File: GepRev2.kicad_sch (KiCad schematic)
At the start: 194 parts

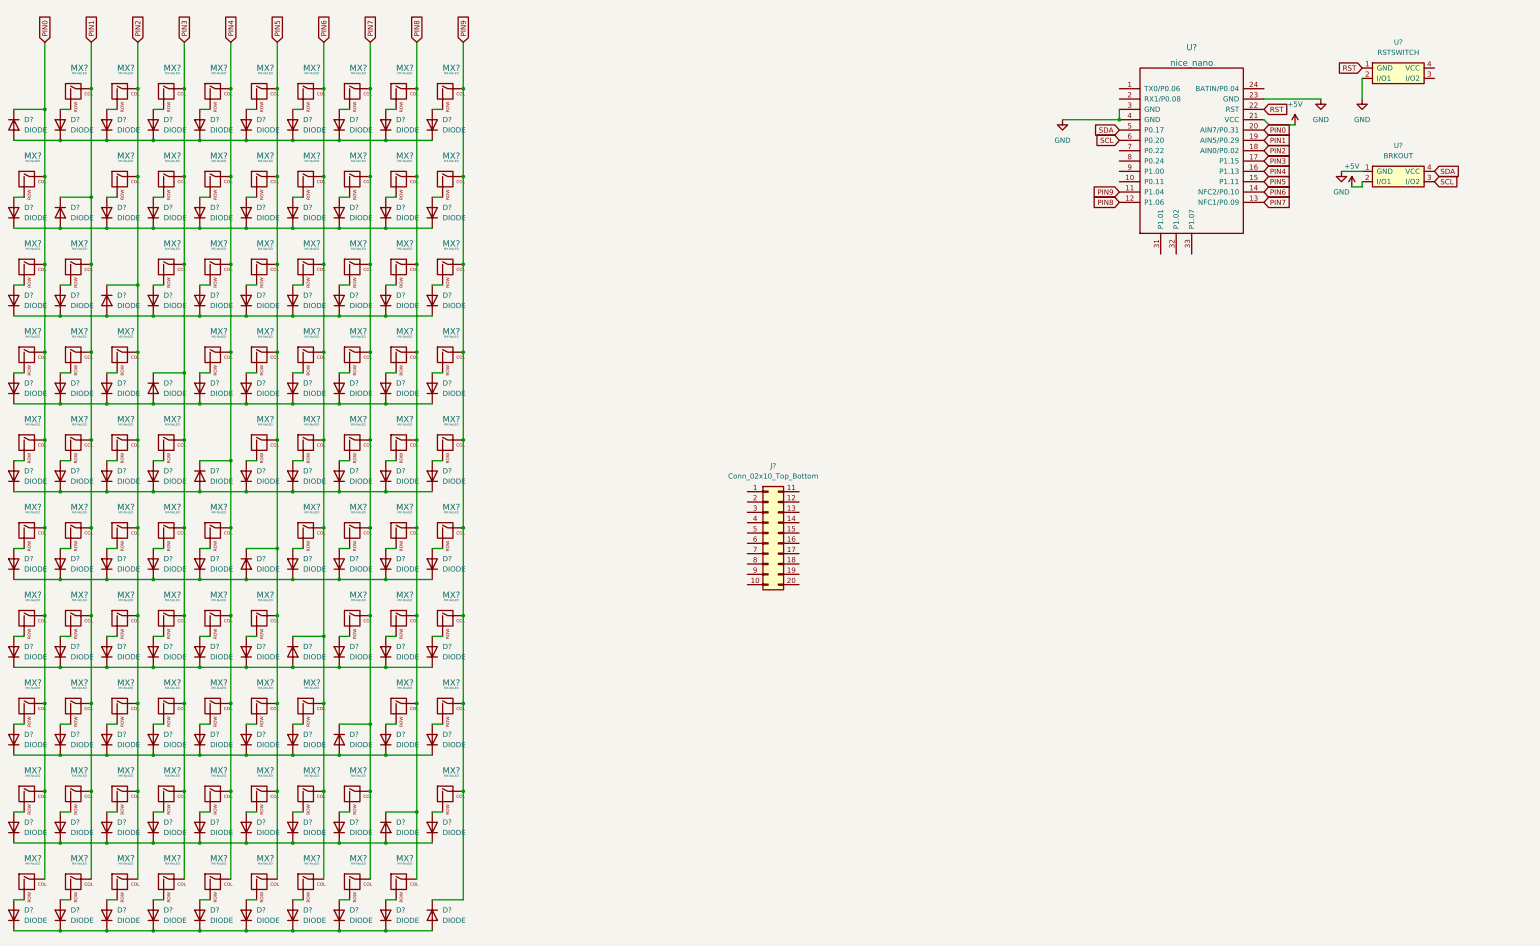
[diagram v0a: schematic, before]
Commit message: Updates to schematic
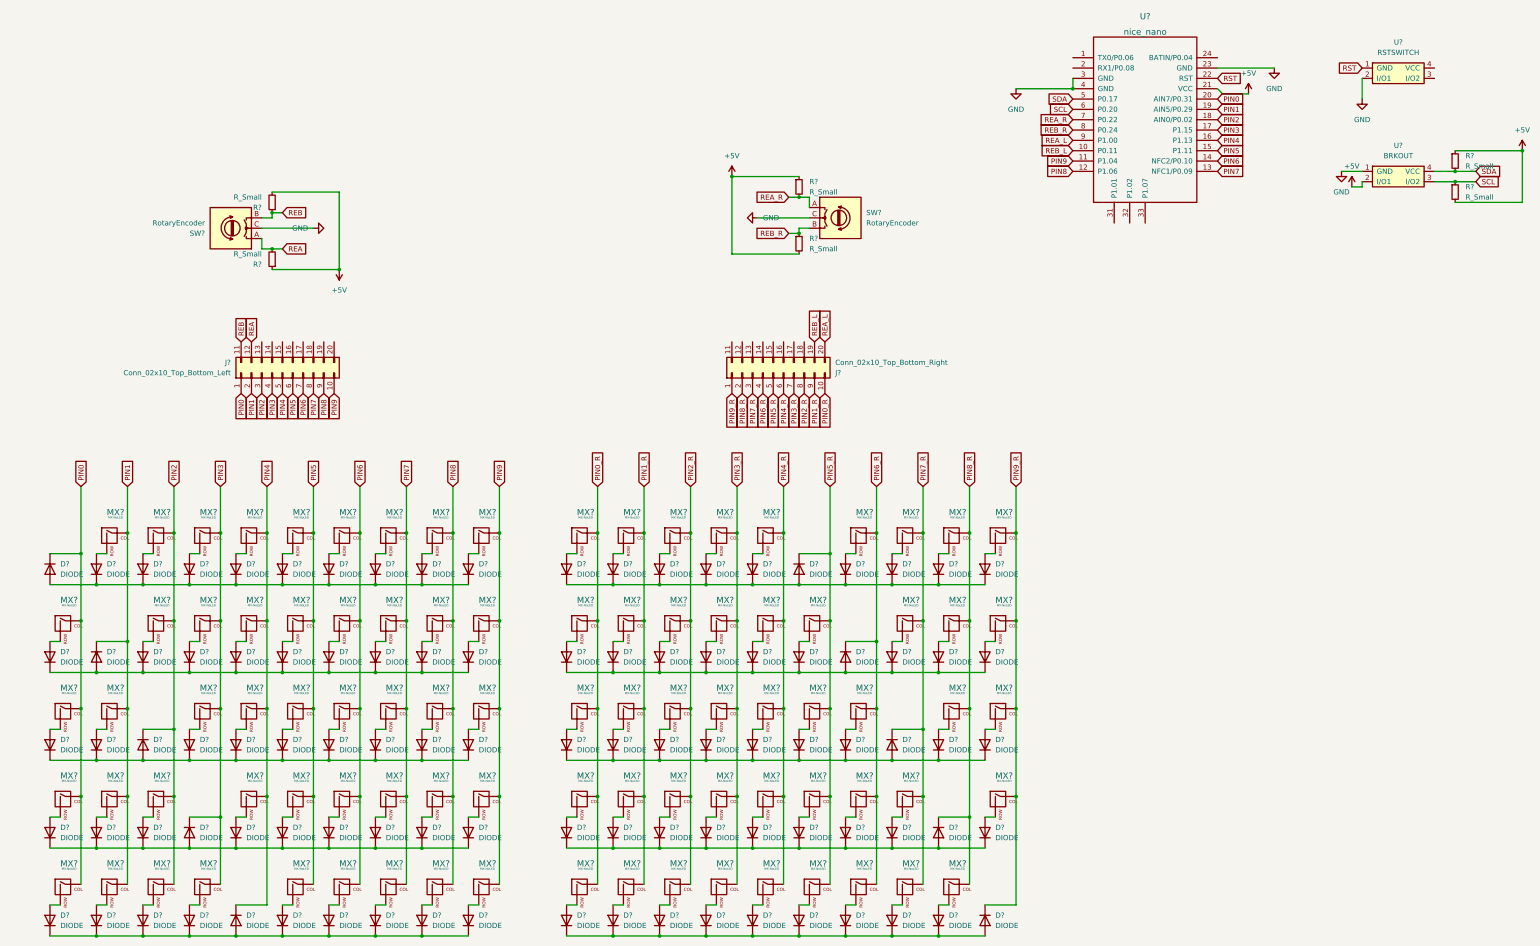
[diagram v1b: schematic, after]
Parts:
- added J?: Conn_02x10_Top_Bottom_Left, symbol Connector_Generic:Conn_02x10_Top_Bottom
- added R? (x6): R_Small, symbol Device:R_Small
- added SW? (x2): RotaryEncoder, symbol Device:RotaryEncoder
- J?: value Conn_02x10_Top_Bottom -> Conn_02x10_Top_Bottom_Right
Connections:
- net +5V: now also R?.1, R?.1, R?.1, R?.2, R?.2, R?.2
- net GND: now also SW?.C, SW?.C
- net PIN0: now also J?.1 (Pin_1); no longer MX?.1 (COL), MX?.1 (COL), MX?.1 (COL), MX?.1 (COL), MX?.1 (COL)
- net PIN1: now also J?.2 (Pin_2); no longer MX?.1 (COL), MX?.1 (COL), MX?.1 (COL), MX?.1 (COL), MX?.1 (COL)
- net PIN2: now also J?.3 (Pin_3); no longer MX?.1 (COL), MX?.1 (COL), MX?.1 (COL), MX?.1 (COL), MX?.1 (COL)
- net PIN3: now also J?.4 (Pin_4); no longer MX?.1 (COL), MX?.1 (COL), MX?.1 (COL), MX?.1 (COL), MX?.1 (COL)
- net PIN4: now also J?.5 (Pin_5); no longer MX?.1 (COL), MX?.1 (COL), MX?.1 (COL), MX?.1 (COL), MX?.1 (COL)
- net PIN5: now also J?.6 (Pin_6); no longer D?.2 (K), MX?.1 (COL), MX?.1 (COL), MX?.1 (COL), MX?.1 (COL)
- net PIN6: now also J?.7 (Pin_7); no longer D?.2 (K), MX?.1 (COL), MX?.1 (COL), MX?.1 (COL), MX?.1 (COL)
- net PIN7: now also J?.8 (Pin_8); no longer D?.2 (K), MX?.1 (COL), MX?.1 (COL), MX?.1 (COL), MX?.1 (COL)
- net PIN8: now also J?.9 (Pin_9); no longer D?.2 (K), MX?.1 (COL), MX?.1 (COL), MX?.1 (COL), MX?.1 (COL)
- net PIN9: now also J?.10 (Pin_10); no longer D?.2 (K), MX?.1 (COL), MX?.1 (COL), MX?.1 (COL), MX?.1 (COL)
- net SCL: now also R?.1
- net SDA: now also R?.2
- net REB_L: now reaches U?.10 (P0.11)
- net REB_L: now also J?.19 (Pin_19)
- net REA_R: now reaches U?.7 (P0.22)
- net REA_R: now also R?.2, SW?.A
- net REB_R: now reaches U?.8 (P0.24)
- net REB_R: now also R?.1, SW?.B
- net REA_L: now reaches U?.9 (P1.00)
- net REA_L: now also J?.20 (Pin_20)
- net PIN9_R: now reaches J?.1 (Pin_1)
- net PIN9_R: now also D?.2 (K), MX?.1 (COL), MX?.1 (COL), MX?.1 (COL), MX?.1 (COL)
- net PIN0_R: now reaches J?.10 (Pin_10)
- net PIN0_R: now also MX?.1 (COL), MX?.1 (COL), MX?.1 (COL), MX?.1 (COL), MX?.1 (COL)
- net PIN8_R: now reaches J?.2 (Pin_2)
- net PIN8_R: now also D?.2 (K), MX?.1 (COL), MX?.1 (COL), MX?.1 (COL), MX?.1 (COL)
- net PIN7_R: now reaches J?.3 (Pin_3)
- net PIN7_R: now also D?.2 (K), MX?.1 (COL), MX?.1 (COL), MX?.1 (COL), MX?.1 (COL)
- net PIN6_R: now reaches J?.4 (Pin_4)
- net PIN6_R: now also D?.2 (K), MX?.1 (COL), MX?.1 (COL), MX?.1 (COL), MX?.1 (COL)
- net PIN5_R: now reaches J?.5 (Pin_5)
- net PIN5_R: now also D?.2 (K), MX?.1 (COL), MX?.1 (COL), MX?.1 (COL), MX?.1 (COL)
- net PIN4_R: now reaches J?.6 (Pin_6)
- net PIN4_R: now also MX?.1 (COL), MX?.1 (COL), MX?.1 (COL), MX?.1 (COL), MX?.1 (COL)
- net PIN3_R: now reaches J?.7 (Pin_7)
- net PIN3_R: now also MX?.1 (COL), MX?.1 (COL), MX?.1 (COL), MX?.1 (COL), MX?.1 (COL)
- net PIN2_R: now reaches J?.8 (Pin_8)
- net PIN2_R: now also MX?.1 (COL), MX?.1 (COL), MX?.1 (COL), MX?.1 (COL), MX?.1 (COL)
- net PIN1_R: now reaches J?.9 (Pin_9)
- net PIN1_R: now also MX?.1 (COL), MX?.1 (COL), MX?.1 (COL), MX?.1 (COL), MX?.1 (COL)
- new net REA: J?.12 (Pin_12), R?.2, SW?.A
- new net REB: J?.11 (Pin_11), R?.1, SW?.B
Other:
- moved on the sheet: D?, J?, MX?, U?
